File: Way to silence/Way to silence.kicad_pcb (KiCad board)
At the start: 2 copper layers, 59.3 x 38.1 mm, 70 parts, among them J1 SD Card Connector, J2 Amplificator_Terminal, J3 5V_Terminal, J4 Battery_Terminal, J6 Conn_01x04_Pin, Q1 BC817, Q2 BC817, SW1 SW_SPDT, SW3 SW_SPST, U1 ESP32-WROOM-32-N16, U2 SM5308, U3 CP2102-GMR, U4 MAX98357AETE+T, U5 USB-TYPE-C-018, U6 AMS1117CD-3.3

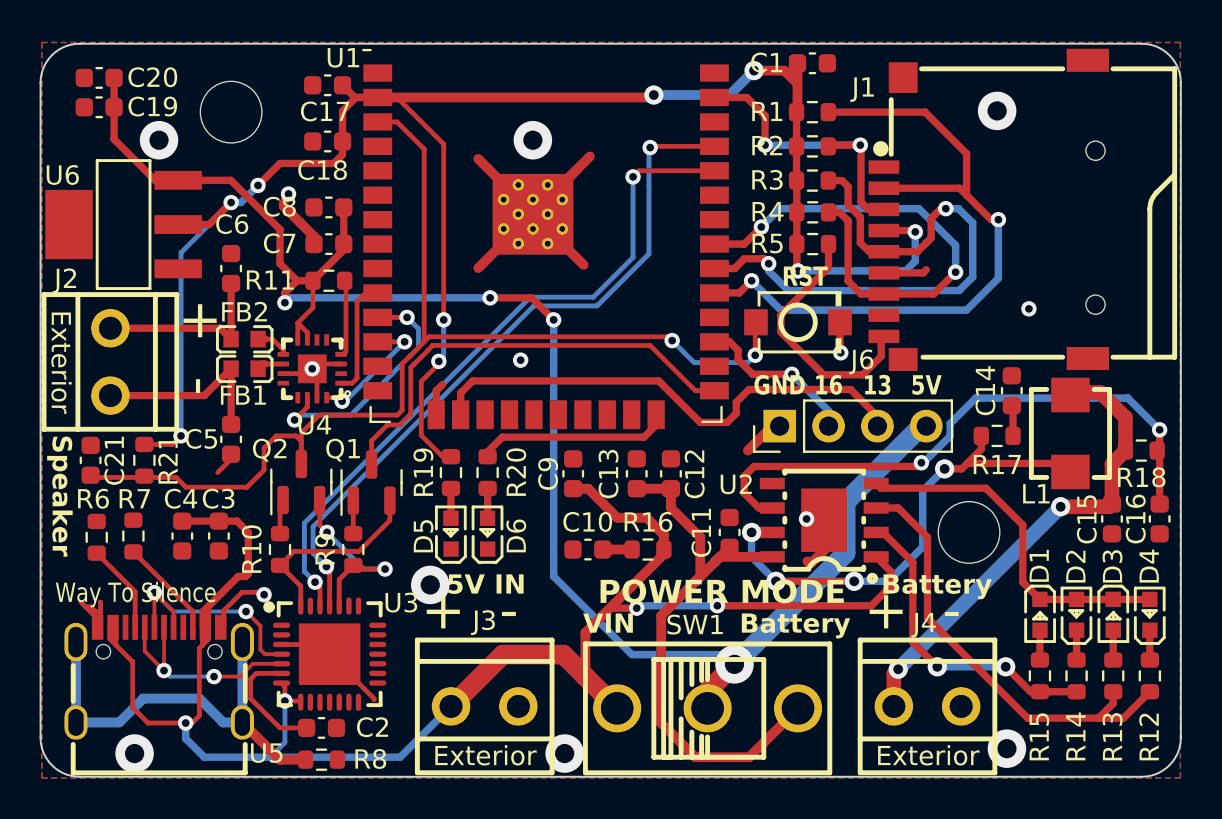
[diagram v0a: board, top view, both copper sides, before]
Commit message: [UDPT] Pcb from schematics
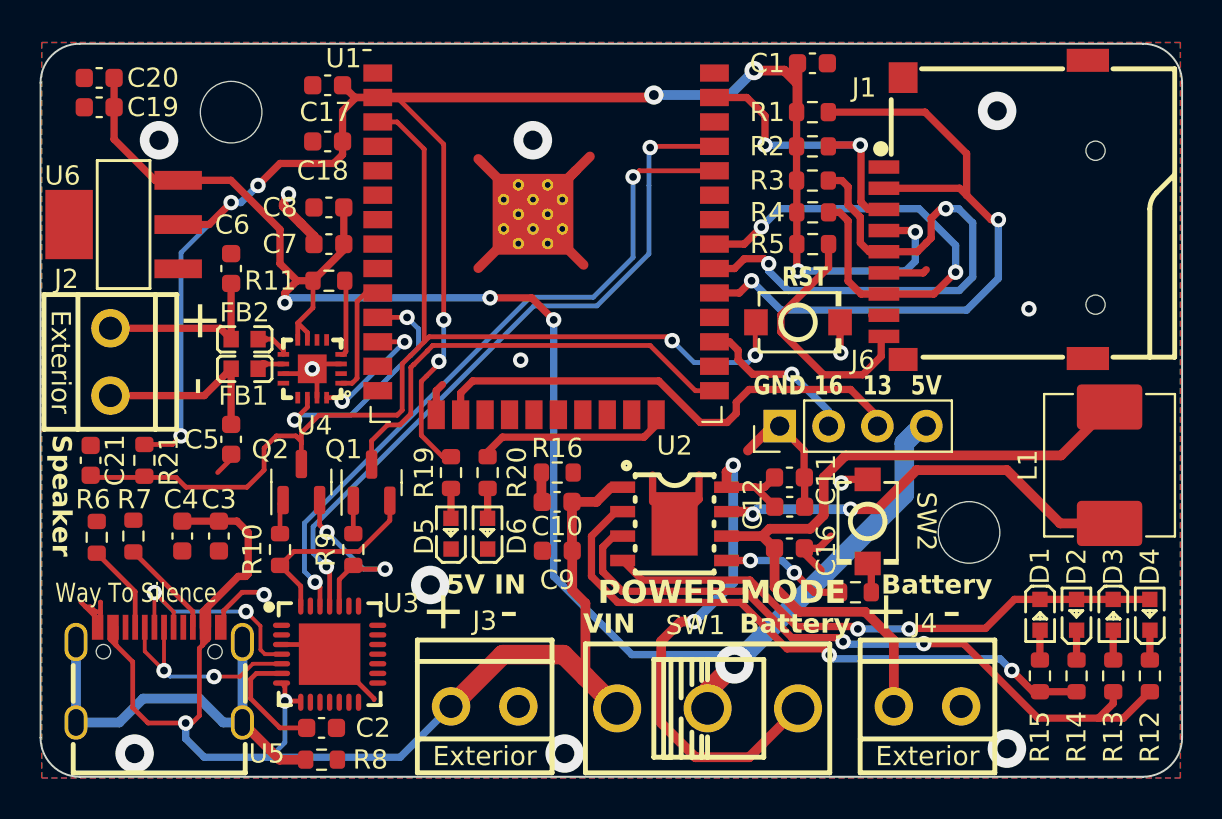
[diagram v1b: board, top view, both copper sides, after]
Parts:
- removed C13, C15: 22uF, Way to silence:C_0603_1608Metric
- removed C14: 4.7nF, Way to silence:C_0603_1608Metric
- removed R18: 0.1R, Way to silence:R_0603_1608Metric
- added SW2: SW_SPST, Way to silence:SW_SPST, F.Cu at (113.7, 76.3)
- C12: value 22uF -> 10uF
- L1: value 1UH -> 2.2UH; footprint Way to silence:Inductor -> Way to silence:Inductor-0630LR
- R16: value 0.5R -> 1R
- R17: value 1R -> 10K
- moved C16 19.3 mm to (109.6, 77.7), turned to 180 degrees
- moved R17 11.0 mm to (113.0, 80.0), turned to 180 degrees
- moved U2 7.78 mm to (103.6, 76.5), turned to 0 degrees
- moved C12 6.41 mm to (109.6, 75.6), turned to 0 degrees
- moved R16 6.18 mm to (97.5, 73.8), turned to 0 degrees
- moved C11 4.22 mm to (109.6, 74.0), turned to 0 degrees
- moved C9 4.08 mm to (97.5, 77.9), turned to 180 degrees
- moved C10 2.95 mm to (97.5, 75.3)
- moved L1 2.62 mm to (126.2, 73.4)
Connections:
- C10 pad 1: Net-(C10-Pad1) -> /USB to Uart/+5V
- C10 pad 2: GND -> Net-(C10-Pad2)
- C16 pad 2: Net-(U2-BAT) -> /BMS/BAT
- R16 pad 1: /USB to Uart/+5V -> Net-(C10-Pad2)
- R16 pad 2: Net-(C10-Pad1) -> GND
- R17 pad 1: Net-(U2-SW) -> Net-(SW2-B)
- R17 pad 2: Net-(C14-Pad1) -> Net-(U2-KEY)
- U2 pad 5: unconnected-(U2-KEY-Pad5) -> Net-(U2-KEY)
- U2 pad 6: Net-(U2-BAT) -> /BMS/BAT
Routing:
- net Net-(U2-BAT): track 30.3 -> 0.00 mm, vias 2 -> 0
- net /USB to Uart/+5V: track 90.6 -> 70.5 mm, vias 4 -> 2
- net Net-(U2-LED1): track 16.3 -> 32.0 mm
- net Net-(U2-LED2): track 23.5 -> 36.4 mm, vias 0 -> 2
- net /BMS/BAT: track 25.0 -> 37.5 mm, vias 2 -> 0
- net Net-(D1-K): track 18.5 -> 29.5 mm, vias 0 -> 2
- net GND: track 76.0 -> 84.9 mm
- net Net-(U2-KEY): track 0.00 -> 6.56 mm, vias 0 -> 2
- net Net-(U2-SW): track 25.7 -> 22.1 mm, vias 4 -> 2
- net Net-(SW2-B): track 0.00 -> 1.58 mm
- net Net-(C10-Pad2): track 0.00 -> 1.54 mm
- net Net-(C14-Pad1): track 1.54 -> 0.00 mm
- net Net-(C10-Pad1): track 1.53 -> 0.00 mm
- net /BMS/VOUT: track 29.9 -> 31.2 mm, vias 0 -> 2
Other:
- outline, holes or cut-outs redrawn
